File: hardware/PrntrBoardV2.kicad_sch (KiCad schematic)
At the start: 13 parts

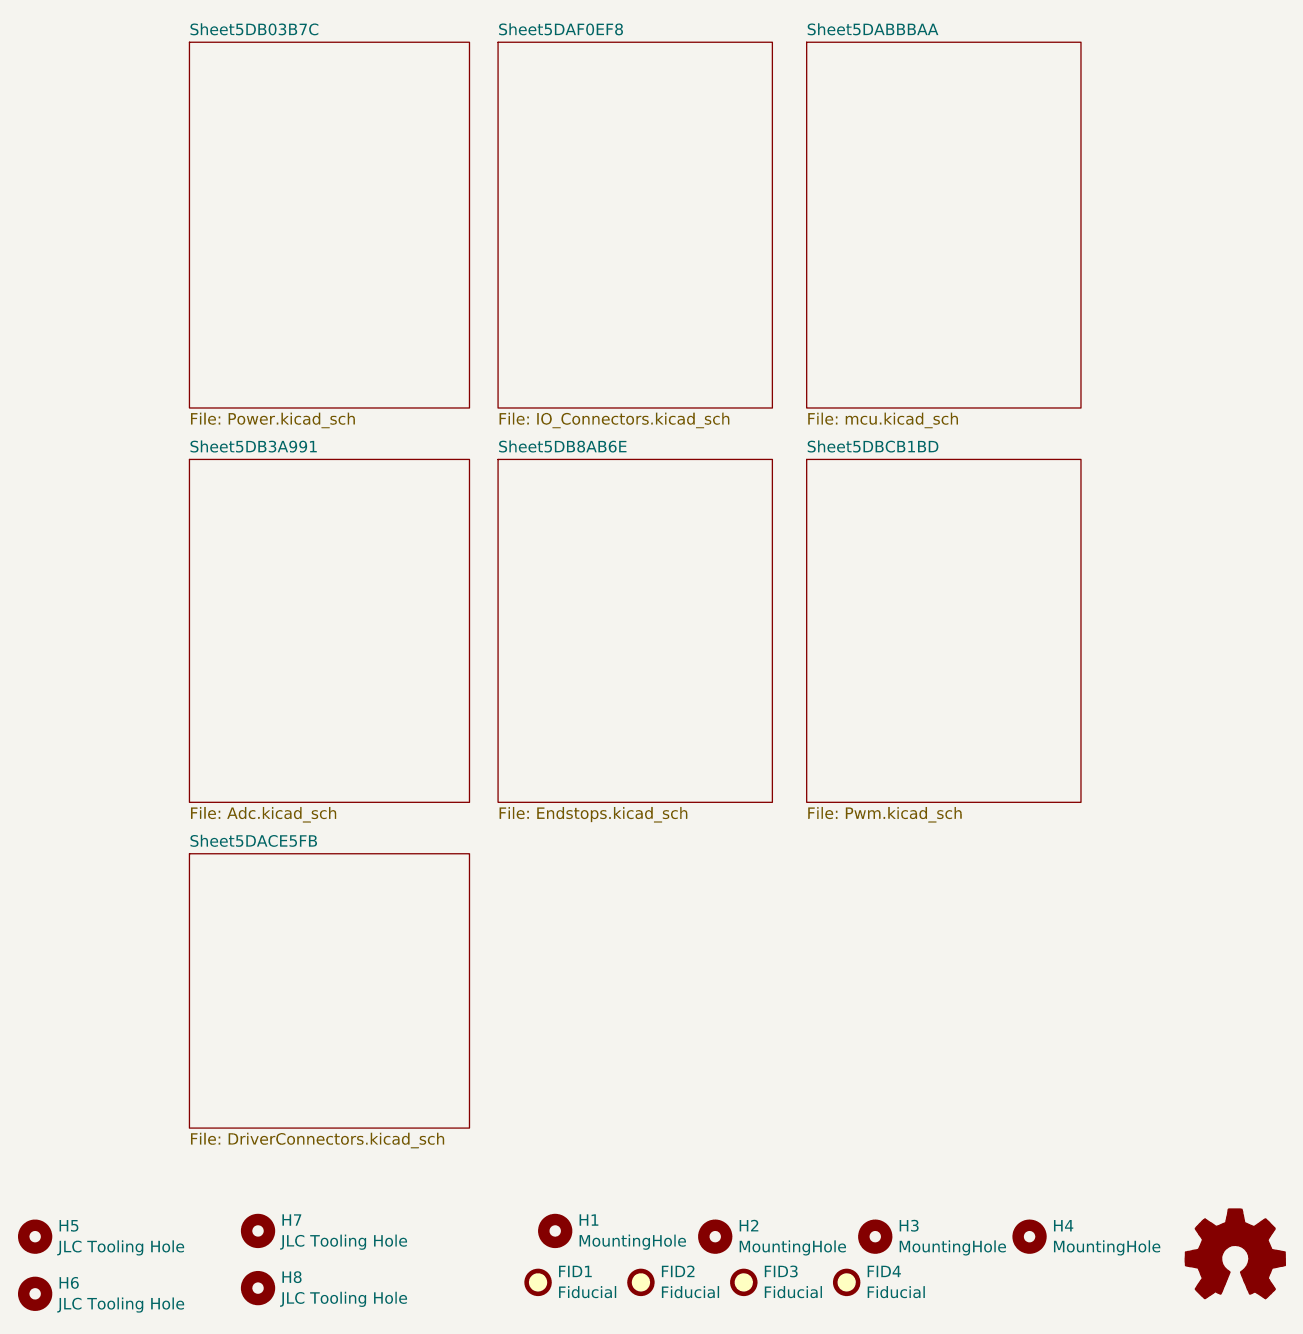
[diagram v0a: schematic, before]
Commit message: Update PrntrBoard fabrication files.
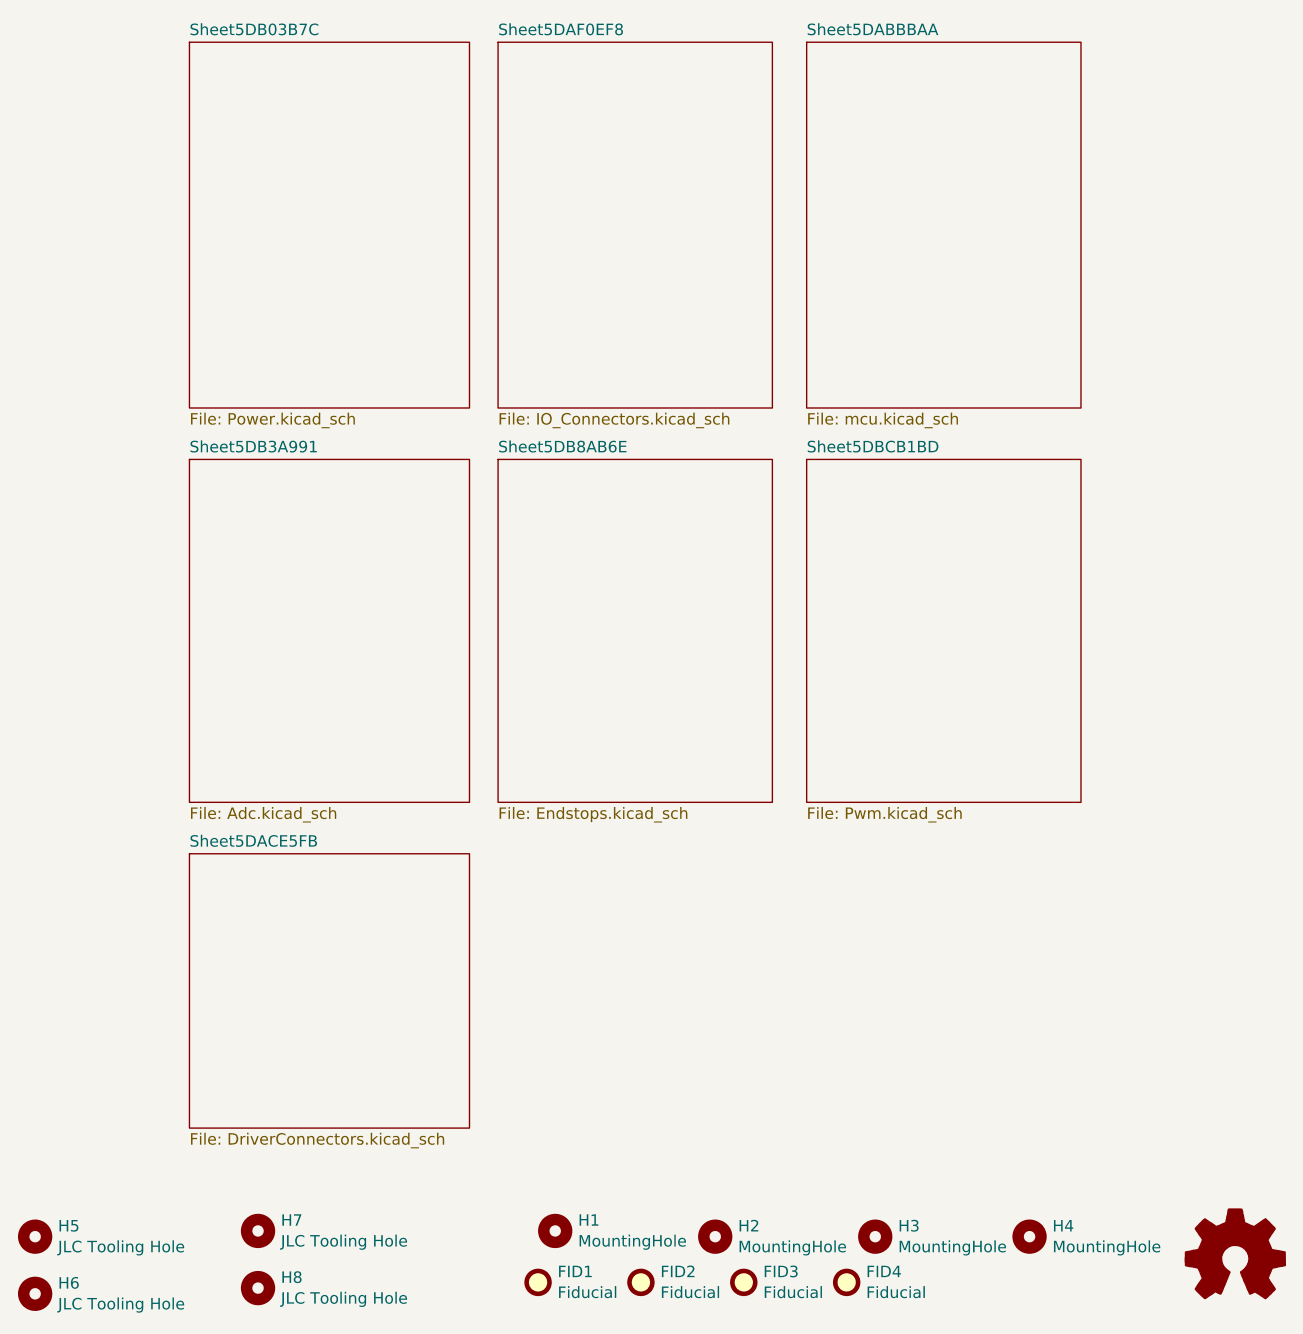
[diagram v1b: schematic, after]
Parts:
- FID1, FID2, FID3, FID4, H1, H2, H3, H4, H5, H6, H7, H8, LOGO1: now left out of the parts list
